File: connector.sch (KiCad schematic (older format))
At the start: 1 part, among them P3 CONN_01X06

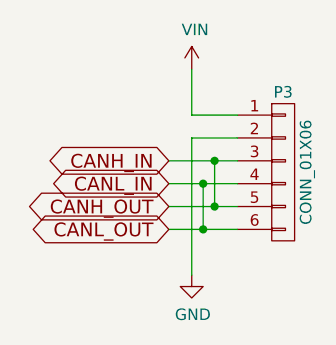
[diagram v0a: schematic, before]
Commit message: Layout: first version
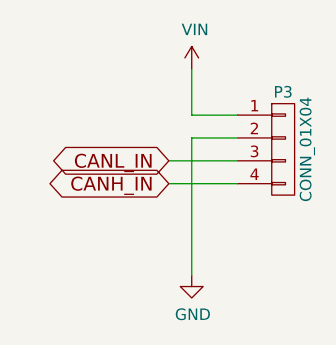
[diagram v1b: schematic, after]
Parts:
- removed P3: CONN_01X06, CAN_Node:WAGO_218-106, symbol CONN_01X06
- added P3: CONN_01X04, CAN_Node:WAGO_218-104, symbol CONN_01X04
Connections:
- net CANH_IN: now also P3.4 (P4)
- net CANL_IN: now also P3.3 (P3)
- net GND: now also P3.2 (P2)
- net VIN: now also P3.1 (P1)
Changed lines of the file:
@@
 $EndDescr
 $Comp
-L GND #PWR054
+L GND #PWR056
 U 1 1 5811BC18
 P 5050 4550
-F 0 "#PWR054" H 5050 4300 50  0001 C CNN
+F 0 "#PWR056" H 5050 4300 50  0001 C CNN
 F 1 "GND" H 5055 4377 50  0000 C CNN
 F 2 "" H 5050 4550 50  0000 C CNN
@@
 	1    0    0    -1
 $EndComp
+Text GLabel 4950 4050 0    60   BiDi ~ 0
+CANL_IN
 Text GLabel 4950 4150 0    60   BiDi ~ 0
-CANL_IN
-Text GLabel 4950 4250 0    60   BiDi ~ 0
-CANH_OUT
-Text GLabel 4950 4350 0    60   BiDi ~ 0
-CANL_OUT
-Text GLabel 4950 4050 0    60   BiDi ~ 0
 CANH_IN
 $Comp
-L VIN #PWR055
+L VIN #PWR057
 U 1 1 5811BC4F
 P 5050 3650
-F 0 "#PWR055" H 5050 3500 50  0001 C CNN
+F 0 "#PWR057" H 5050 3500 50  0001 C CNN
 F 1 "VIN" H 5065 3823 50  0000 C CNN
 F 2 "" H 5050 3650 60  0000 C CNN
@@
 Wire Wire Line
 	4950 4150 5250 4150
-Wire Wire Line
-	4950 4250 5250 4250
-Wire Wire Line
-	4950 4350 5250 4350
 Wire Wire Line
 	5050 4550 5050 3950
@@
 Wire Wire Line
 	4950 4050 5250 4050
-Wire Wire Line
-	5100 4150 5100 4350
-Connection ~ 5100 4350
-Connection ~ 5100 4150
-Wire Wire Line
-	5150 4250 5150 4050
-Connection ~ 5150 4050
-Connection ~ 5150 4250
 $Comp
-L CONN_01X06 P3
-U 1 1 58146F94
-P 5450 4100
-F 0 "P3" H 5450 4450 50  0000 C CNN
-F 1 "CONN_01X06" V 5550 4100 50  0000 C CNN
-F 2 "CAN_Node:WAGO_218-106" H 5450 4100 50  0001 C CNN
-F 3 "" H 5450 4100 50  0000 C CNN
-	1    5450 4100
+L CONN_01X04 P3
+U 1 1 581AFCAF
+P 5450 4000
+F 0 "P3" H 5450 4250 50  0000 C CNN
+F 1 "CONN_01X04" V 5550 4000 50  0000 C CNN
+F 2 "CAN_Node:WAGO_218-104" H 5450 4000 50  0001 C CNN
+F 3 "" H 5450 4000 50  0000 C CNN
+	1    5450 4000
 	1    0    0    -1
 $EndComp
